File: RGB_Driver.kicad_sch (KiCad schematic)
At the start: 2 parts, among them U13 IS31FL3729-QF, U9 IS31FL3729-QF

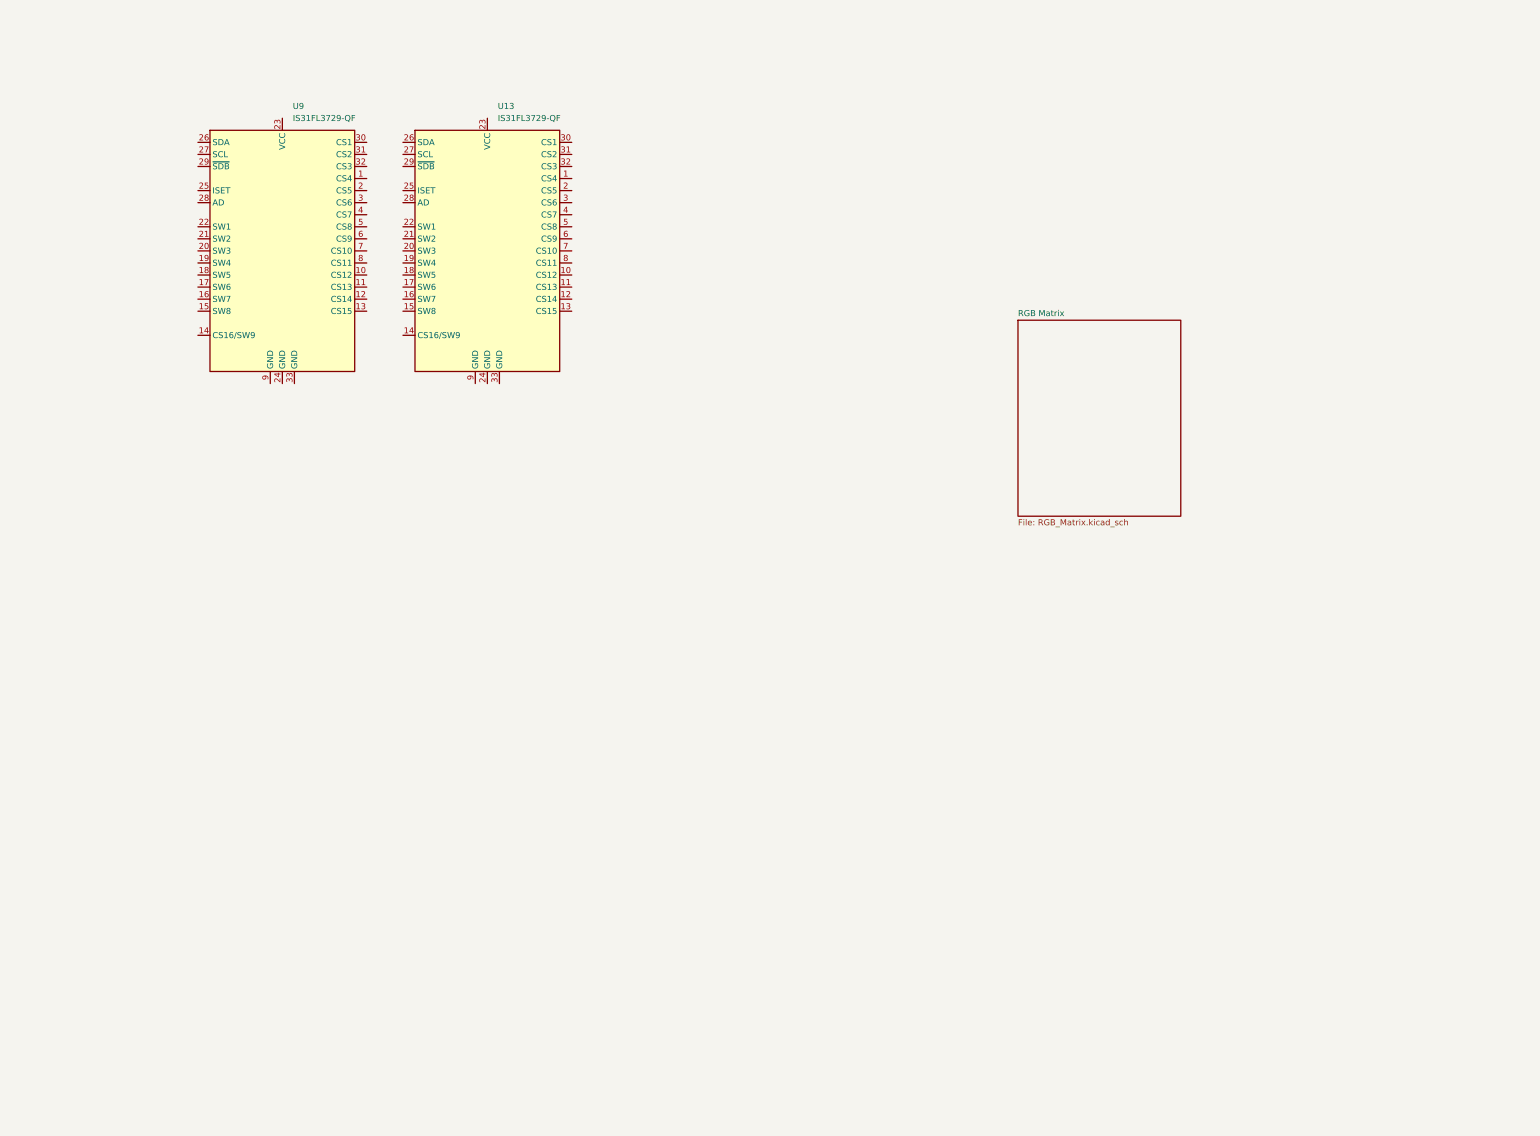
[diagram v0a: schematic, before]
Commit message: Change
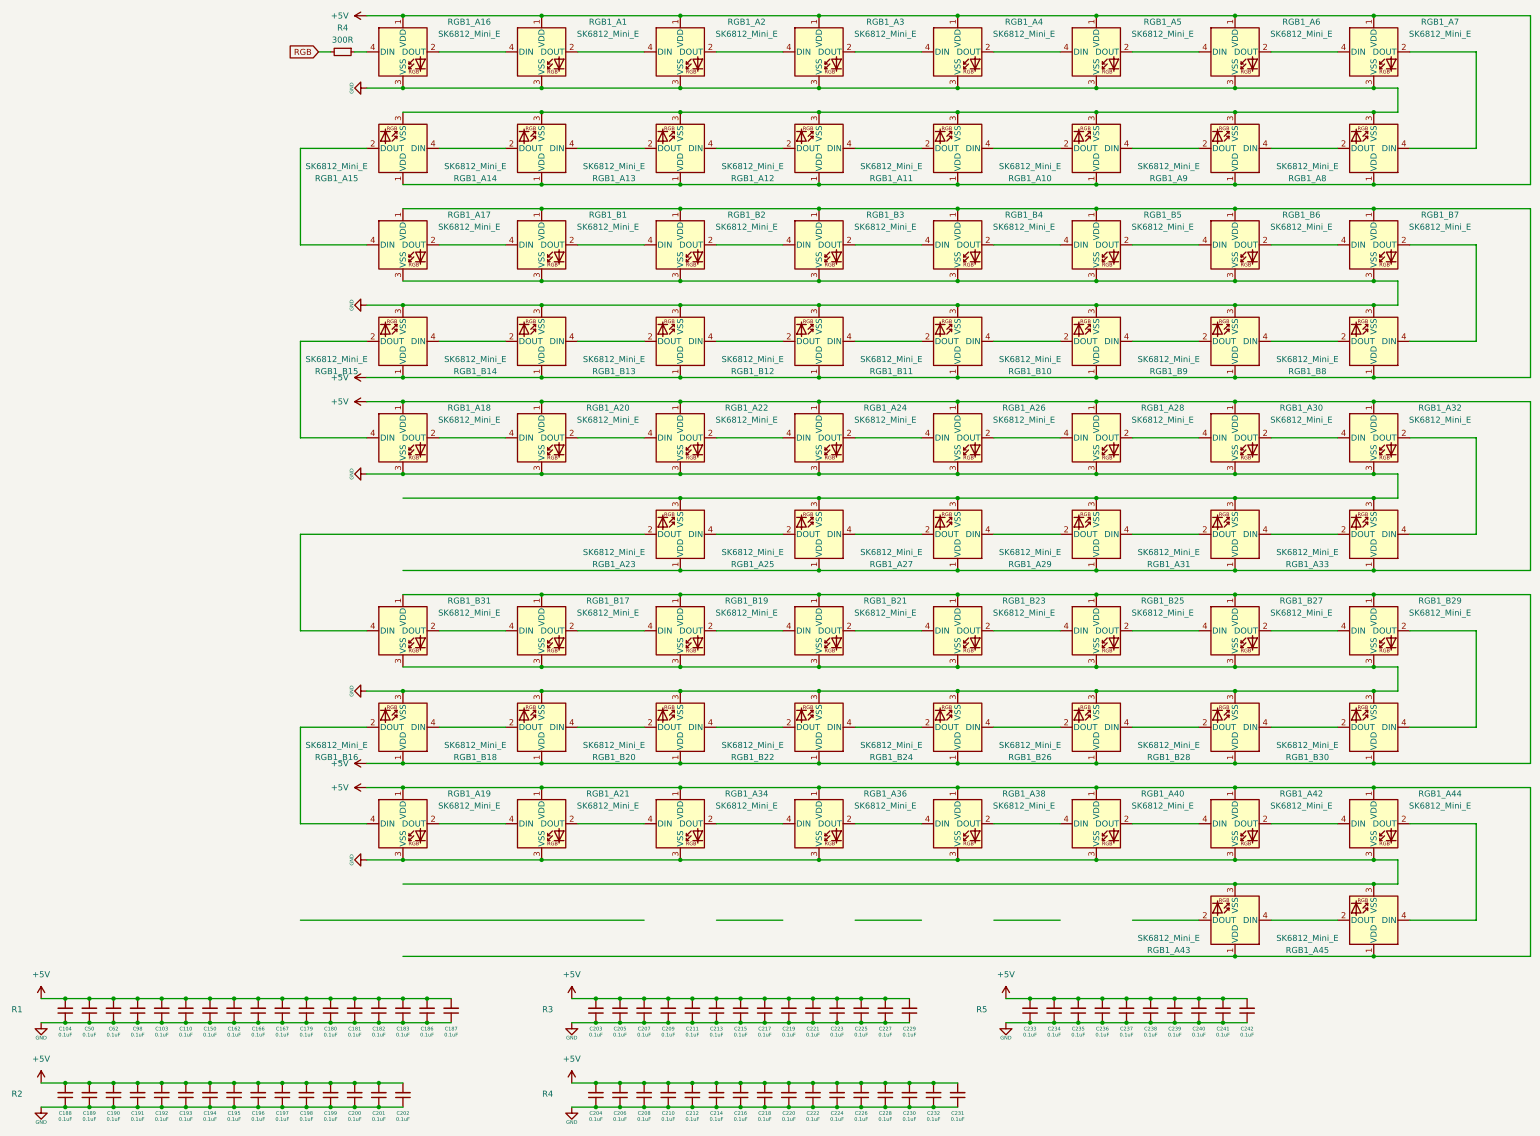
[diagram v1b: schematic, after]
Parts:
- removed U13, U9: IS31FL3729-QF, Package_DFN_QFN:QFN-32-1EP_4x4mm_P0.4mm_EP2.9x2.9mm_ThermalVias, symbol horrortroll_lib:IS31FL3729-QF
- added C103, C104, C110, C150, C162, C166, C167, C179, C180, C181, C182, C183, C186, C187, C188, C189, C190, C191, C192, C193, C194, C195, C196, C197, C198, C199, C200, C201, C202, C203, C204, C205, C206, C207, C208, C209, C210, C211, C212, C213, C214, C215, C216, C217, C218, C219, C220, C221, C222, C223, C224, C225, C226, C227, C228, C229, C230, C231, C232, C233, C234, C235, C236, C237, C238, C239, C240, C241, C242, C50, C62, C98: 0.1uF, Common_Footprint:C_0603, symbol Device:C_Small
- added R4: 300R, Common_Footprint:R_0402, symbol Device:R_Small
- added RGB1_A1, RGB1_A10, RGB1_A11, RGB1_A12, RGB1_A13, RGB1_A14, RGB1_A15, RGB1_A16, RGB1_A17, RGB1_A18, RGB1_A19, RGB1_A2, RGB1_A20, RGB1_A21, RGB1_A22, RGB1_A23, RGB1_A24, RGB1_A25, RGB1_A26, RGB1_A27, RGB1_A28, RGB1_A29, RGB1_A3, RGB1_A30, RGB1_A31, RGB1_A32, RGB1_A33, RGB1_A34, RGB1_A36, RGB1_A38, RGB1_A4, RGB1_A40, RGB1_A42, RGB1_A43, RGB1_A44, RGB1_A45, RGB1_A5, RGB1_A6, RGB1_A7, RGB1_A8, RGB1_A9: SK6812_Mini_E, RGB_Addressable:SK6812_Mini_E_REV, symbol Salane Personal Symbol:SK6812_Mini_E
- added RGB1_B1, RGB1_B10, RGB1_B11, RGB1_B12, RGB1_B13, RGB1_B14, RGB1_B15, RGB1_B16, RGB1_B17, RGB1_B18, RGB1_B19, RGB1_B2, RGB1_B20, RGB1_B21, RGB1_B22, RGB1_B23, RGB1_B24, RGB1_B25, RGB1_B26, RGB1_B27, RGB1_B28, RGB1_B29, RGB1_B3, RGB1_B30, RGB1_B31, RGB1_B4, RGB1_B5, RGB1_B6, RGB1_B7, RGB1_B8, RGB1_B9: SK6812_Mini_E, RGB_Addressable:SK6812_Mini_E, symbol Salane Personal Symbol:SK6812_Mini_E
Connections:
- new net: RGB1_B24.4 (DIN), RGB1_B26.2 (DOUT)
- new net: RGB1_B26.4 (DIN), RGB1_B28.2 (DOUT)
- new net: RGB1_B12.2 (DOUT), RGB1_B13.4 (DIN)
- new net: RGB1_B11.2 (DOUT), RGB1_B12.4 (DIN)
- new net: RGB1_B6.2 (DOUT), RGB1_B7.4 (DIN)
- new net: RGB1_B5.2 (DOUT), RGB1_B6.4 (DIN)
- new net: RGB1_A2.2 (DOUT), RGB1_A3.4 (DIN)
- new net: RGB1_A1.2 (DOUT), RGB1_A2.4 (DIN)
- new net: RGB1_A4.2 (DOUT), RGB1_A5.4 (DIN)
- new net: RGB1_A3.2 (DOUT), RGB1_A4.4 (DIN)
- new net: RGB1_A15.2 (DOUT), RGB1_A17.4 (DIN)
- new net: RGB1_A14.2 (DOUT), RGB1_A15.4 (DIN)
- new net: RGB1_B22.4 (DIN), RGB1_B24.2 (DOUT)
- new net: RGB1_A5.2 (DOUT), RGB1_A6.4 (DIN)
- new net: RGB1_A42.2 (DOUT), RGB1_A44.4 (DIN)
- new net: RGB1_A40.2 (DOUT), RGB1_A42.4 (DIN)
- new net: RGB1_A17.2 (DOUT), RGB1_B1.4 (DIN)
- new net: RGB1_B1.2 (DOUT), RGB1_B2.4 (DIN)
- new net: RGB1_A25.4 (DIN), RGB1_A27.2 (DOUT)
- new net: RGB1_A27.4 (DIN), RGB1_A29.2 (DOUT)
- new net: RGB1_B21.2 (DOUT), RGB1_B23.4 (DIN)
- new net: RGB1_B19.2 (DOUT), RGB1_B21.4 (DIN)
- new net: RGB1_B18.4 (DIN), RGB1_B20.2 (DOUT)
- new net: RGB1_B20.4 (DIN), RGB1_B22.2 (DOUT)
- new net: RGB1_B10.4 (DIN), RGB1_B9.2 (DOUT)
- new net: RGB1_B8.2 (DOUT), RGB1_B9.4 (DIN)
- new net: RGB1_A34.2 (DOUT), RGB1_A36.4 (DIN)
- new net: RGB1_A21.2 (DOUT), RGB1_A34.4 (DIN)
- new net: RGB1_A29.4 (DIN), RGB1_A31.2 (DOUT)
- new net: RGB1_A7.2 (DOUT), RGB1_A8.4 (DIN)
- new net: RGB1_A6.2 (DOUT), RGB1_A7.4 (DIN)
- new net: RGB1_A19.4 (DIN), RGB1_B16.2 (DOUT)
- new net: RGB1_B16.4 (DIN), RGB1_B18.2 (DOUT)
- new net: RGB1_B2.2 (DOUT), RGB1_B3.4 (DIN)
- new net: RGB1_B3.2 (DOUT), RGB1_B4.4 (DIN)
- new net: RGB1_A43.4 (DIN), RGB1_A45.2 (DOUT)
- new net: RGB1_A38.2 (DOUT), RGB1_A40.4 (DIN)
- new net: RGB1_A36.2 (DOUT), RGB1_A38.4 (DIN)
- new net: RGB1_A24.2 (DOUT), RGB1_A26.4 (DIN)
- new net: RGB1_A22.2 (DOUT), RGB1_A24.4 (DIN)
- new net: R4.1, RGB1_A16.4 (DIN)
- new net: RGB1_A30.2 (DOUT), RGB1_A32.4 (DIN)
- new net: RGB1_A28.2 (DOUT), RGB1_A30.4 (DIN)
- new net: RGB1_B10.2 (DOUT), RGB1_B11.4 (DIN)
- new net: RGB1_B28.4 (DIN), RGB1_B30.2 (DOUT)
- new net: RGB1_B29.2 (DOUT), RGB1_B30.4 (DIN)
- new net: RGB1_A13.2 (DOUT), RGB1_A14.4 (DIN)
- new net: RGB1_A12.2 (DOUT), RGB1_A13.4 (DIN)
- new net: RGB1_A11.2 (DOUT), RGB1_A12.4 (DIN)
- new net: RGB1_B27.2 (DOUT), RGB1_B29.4 (DIN)
- new net: RGB1_B25.2 (DOUT), RGB1_B27.4 (DIN)
- new net: RGB1_B7.2 (DOUT), RGB1_B8.4 (DIN)
- new net: RGB1_A18.4 (DIN), RGB1_B15.2 (DOUT)
- new net: RGB1_B14.2 (DOUT), RGB1_B15.4 (DIN)
- new net: RGB1_A32.2 (DOUT), RGB1_A33.4 (DIN)
- new net: RGB1_B13.2 (DOUT), RGB1_B14.4 (DIN)
- new net: RGB1_A31.4 (DIN), RGB1_A33.2 (DOUT)
- new net: RGB1_A1.4 (DIN), RGB1_A16.2 (DOUT)
- new net: RGB1_A8.2 (DOUT), RGB1_A9.4 (DIN)
- new net: RGB1_B17.2 (DOUT), RGB1_B19.4 (DIN)
- new net: RGB1_B17.4 (DIN), RGB1_B31.2 (DOUT)
- new net: RGB1_A23.4 (DIN), RGB1_A25.2 (DOUT)
- new net: RGB1_A10.2 (DOUT), RGB1_A11.4 (DIN)
- new net: RGB1_B4.2 (DOUT), RGB1_B5.4 (DIN)
- new net: RGB1_A44.2 (DOUT), RGB1_A45.4 (DIN)
- new net: RGB1_A10.4 (DIN), RGB1_A9.2 (DOUT)
- new net: RGB1_A23.2 (DOUT), RGB1_B31.4 (DIN)
- new net: RGB1_A20.2 (DOUT), RGB1_A22.4 (DIN)
- new net: RGB1_A18.2 (DOUT), RGB1_A20.4 (DIN)
- new net: RGB1_A19.2 (DOUT), RGB1_A21.4 (DIN)
- new net: RGB1_A26.2 (DOUT), RGB1_A28.4 (DIN)
- new net: RGB1_B23.2 (DOUT), RGB1_B25.4 (DIN)
- new net +5V: C103.2, C104.2, C110.2, C150.2, C162.2, C166.2, C167.2, C179.2, C180.2, C181.2, C182.2, C183.2, C186.2, C187.2, C188.2, C189.2, C190.2, C191.2, C192.2, C193.2, C194.2, C195.2, C196.2, C197.2, C198.2, C199.2, C200.2, C201.2, C202.2, C203.2, C204.2, C205.2, C206.2, C207.2, C208.2, C209.2, C210.2, C211.2, C212.2, C213.2, C214.2, C215.2, C216.2, C217.2, C218.2, C219.2, C220.2, C221.2, C222.2, C223.2, C224.2, C225.2, C226.2, C227.2, C228.2, C229.2, C230.2, C231.2, C232.2, C233.2, C234.2, C235.2, C236.2, C237.2, C238.2, C239.2, C240.2, C241.2, C242.2, C50.2, C62.2, C98.2, RGB1_A1.1 (VDD), RGB1_A10.1 (VDD), RGB1_A11.1 (VDD), RGB1_A12.1 (VDD), RGB1_A13.1 (VDD), RGB1_A14.1 (VDD), RGB1_A15.1 (VDD), RGB1_A16.1 (VDD), RGB1_A17.1 (VDD), RGB1_A18.1 (VDD), RGB1_A19.1 (VDD), RGB1_A2.1 (VDD), RGB1_A20.1 (VDD), RGB1_A21.1 (VDD), RGB1_A22.1 (VDD), RGB1_A23.1 (VDD), RGB1_A24.1 (VDD), RGB1_A25.1 (VDD), RGB1_A26.1 (VDD), RGB1_A27.1 (VDD), RGB1_A28.1 (VDD), RGB1_A29.1 (VDD), RGB1_A3.1 (VDD), RGB1_A30.1 (VDD), RGB1_A31.1 (VDD), RGB1_A32.1 (VDD), RGB1_A33.1 (VDD), RGB1_A34.1 (VDD), RGB1_A36.1 (VDD), RGB1_A38.1 (VDD), RGB1_A4.1 (VDD), RGB1_A40.1 (VDD), RGB1_A42.1 (VDD), RGB1_A43.1 (VDD), RGB1_A44.1 (VDD), RGB1_A45.1 (VDD), RGB1_A5.1 (VDD), RGB1_A6.1 (VDD), RGB1_A7.1 (VDD), RGB1_A8.1 (VDD), RGB1_A9.1 (VDD), RGB1_B1.1 (VDD), RGB1_B10.1 (VDD), RGB1_B11.1 (VDD), RGB1_B12.1 (VDD), RGB1_B13.1 (VDD), RGB1_B14.1 (VDD), RGB1_B15.1 (VDD), RGB1_B16.1 (VDD), RGB1_B17.1 (VDD), RGB1_B18.1 (VDD), RGB1_B19.1 (VDD), RGB1_B2.1 (VDD), RGB1_B20.1 (VDD), RGB1_B21.1 (VDD), RGB1_B22.1 (VDD), RGB1_B23.1 (VDD), RGB1_B24.1 (VDD), RGB1_B25.1 (VDD), RGB1_B26.1 (VDD), RGB1_B27.1 (VDD), RGB1_B28.1 (VDD), RGB1_B29.1 (VDD), RGB1_B3.1 (VDD), RGB1_B30.1 (VDD), RGB1_B31.1 (VDD), RGB1_B4.1 (VDD), RGB1_B5.1 (VDD), RGB1_B6.1 (VDD), RGB1_B7.1 (VDD), RGB1_B8.1 (VDD), RGB1_B9.1 (VDD)
- new net GND: C103.1, C104.1, C110.1, C150.1, C162.1, C166.1, C167.1, C179.1, C180.1, C181.1, C182.1, C183.1, C186.1, C187.1, C188.1, C189.1, C190.1, C191.1, C192.1, C193.1, C194.1, C195.1, C196.1, C197.1, C198.1, C199.1, C200.1, C201.1, C202.1, C203.1, C204.1, C205.1, C206.1, C207.1, C208.1, C209.1, C210.1, C211.1, C212.1, C213.1, C214.1, C215.1, C216.1, C217.1, C218.1, C219.1, C220.1, C221.1, C222.1, C223.1, C224.1, C225.1, C226.1, C227.1, C228.1, C229.1, C230.1, C231.1, C232.1, C233.1, C234.1, C235.1, C236.1, C237.1, C238.1, C239.1, C240.1, C241.1, C242.1, C50.1, C62.1, C98.1, RGB1_A1.3 (VSS), RGB1_A10.3 (VSS), RGB1_A11.3 (VSS), RGB1_A12.3 (VSS), RGB1_A13.3 (VSS), RGB1_A14.3 (VSS), RGB1_A15.3 (VSS), RGB1_A16.3 (VSS), RGB1_A17.3 (VSS), RGB1_A18.3 (VSS), RGB1_A19.3 (VSS), RGB1_A2.3 (VSS), RGB1_A20.3 (VSS), RGB1_A21.3 (VSS), RGB1_A22.3 (VSS), RGB1_A23.3 (VSS), RGB1_A24.3 (VSS), RGB1_A25.3 (VSS), RGB1_A26.3 (VSS), RGB1_A27.3 (VSS), RGB1_A28.3 (VSS), RGB1_A29.3 (VSS), RGB1_A3.3 (VSS), RGB1_A30.3 (VSS), RGB1_A31.3 (VSS), RGB1_A32.3 (VSS), RGB1_A33.3 (VSS), RGB1_A34.3 (VSS), RGB1_A36.3 (VSS), RGB1_A38.3 (VSS), RGB1_A4.3 (VSS), RGB1_A40.3 (VSS), RGB1_A42.3 (VSS), RGB1_A43.3 (VSS), RGB1_A44.3 (VSS), RGB1_A45.3 (VSS), RGB1_A5.3 (VSS), RGB1_A6.3 (VSS), RGB1_A7.3 (VSS), RGB1_A8.3 (VSS), RGB1_A9.3 (VSS), RGB1_B1.3 (VSS), RGB1_B10.3 (VSS), RGB1_B11.3 (VSS), RGB1_B12.3 (VSS), RGB1_B13.3 (VSS), RGB1_B14.3 (VSS), RGB1_B15.3 (VSS), RGB1_B16.3 (VSS), RGB1_B17.3 (VSS), RGB1_B18.3 (VSS), RGB1_B19.3 (VSS), RGB1_B2.3 (VSS), RGB1_B20.3 (VSS), RGB1_B21.3 (VSS), RGB1_B22.3 (VSS), RGB1_B23.3 (VSS), RGB1_B24.3 (VSS), RGB1_B25.3 (VSS), RGB1_B26.3 (VSS), RGB1_B27.3 (VSS), RGB1_B28.3 (VSS), RGB1_B29.3 (VSS), RGB1_B3.3 (VSS), RGB1_B30.3 (VSS), RGB1_B31.3 (VSS), RGB1_B4.3 (VSS), RGB1_B5.3 (VSS), RGB1_B6.3 (VSS), RGB1_B7.3 (VSS), RGB1_B8.3 (VSS), RGB1_B9.3 (VSS)
- new net RGB: R4.2
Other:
- removed sheet RGB Matrix
- note added: "R1"
- note added: "R2"
- note added: "R3"
- note added: "R4"
- note added: "R5"
